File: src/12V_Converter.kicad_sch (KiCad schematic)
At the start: 37 parts, among them M4 CSD19534Q5A, M5 NVMFS6H836NLT1G, U2 LM5190RGYR (20V-50V)

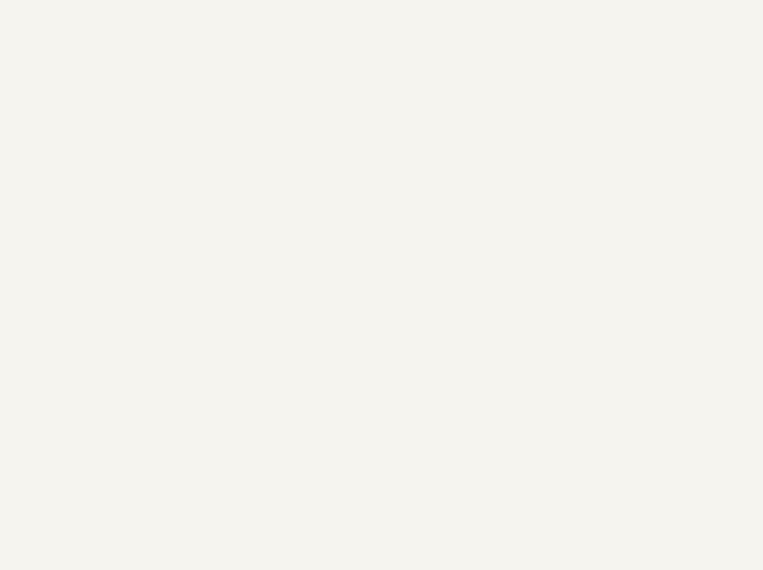
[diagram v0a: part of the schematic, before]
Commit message: Testing once again
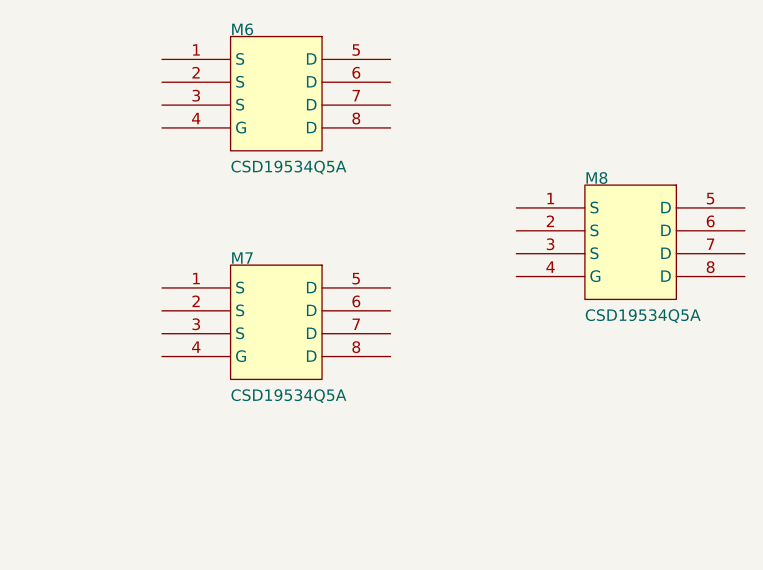
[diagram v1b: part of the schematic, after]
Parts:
- added M6, M7, M8: CSD19534Q5A, powerDristributionBoard-import-fps:DQJ8, symbol Schlib1:CSD19534Q5A

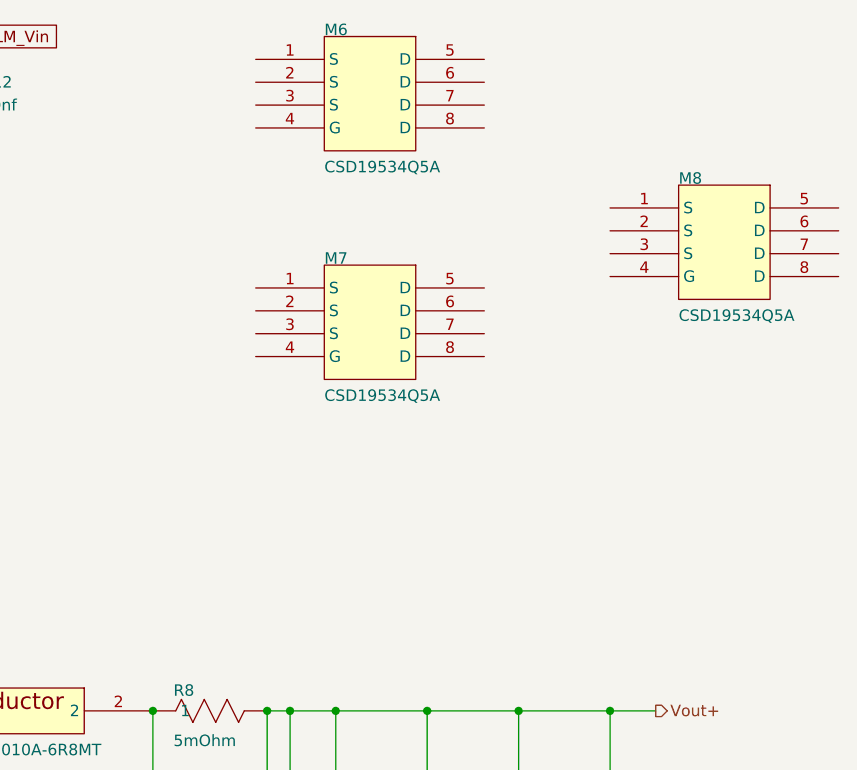
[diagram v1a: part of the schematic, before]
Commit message: Restored powerDistribution PCB files to commit 2fb1c3a
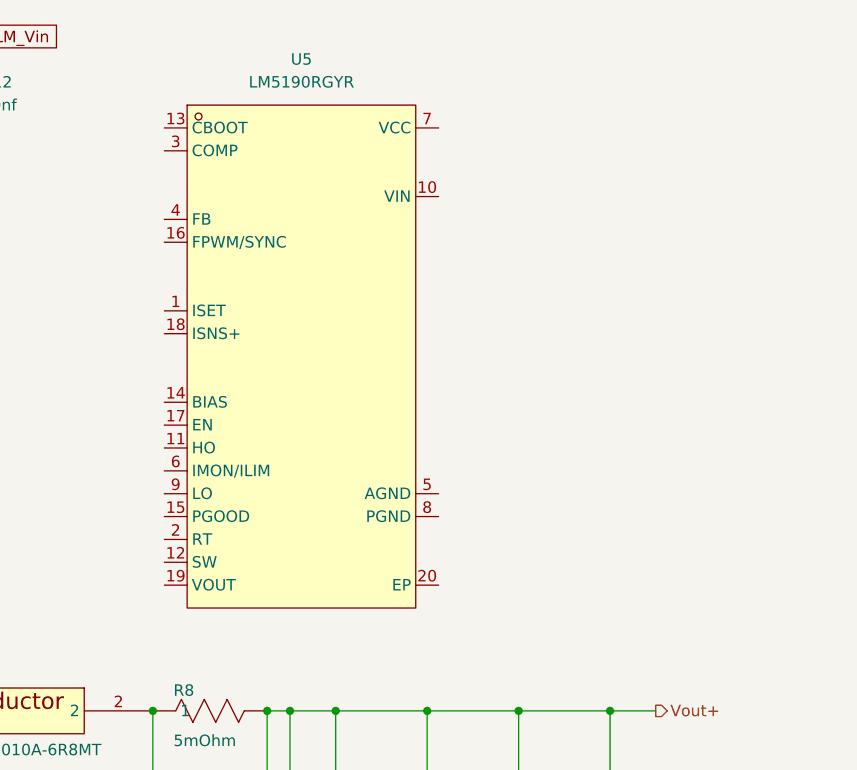
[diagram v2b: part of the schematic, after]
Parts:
- removed M6, M7, M8: CSD19534Q5A, powerDristributionBoard-import-fps:DQJ8, symbol Schlib1:CSD19534Q5A
- added U5: LM5190RGYR, EasyEDA:QFN-19_L4.5-W3.5-P0.50-BL-EP_TI_RGY, symbol EasyEDA:LM5190RGYR

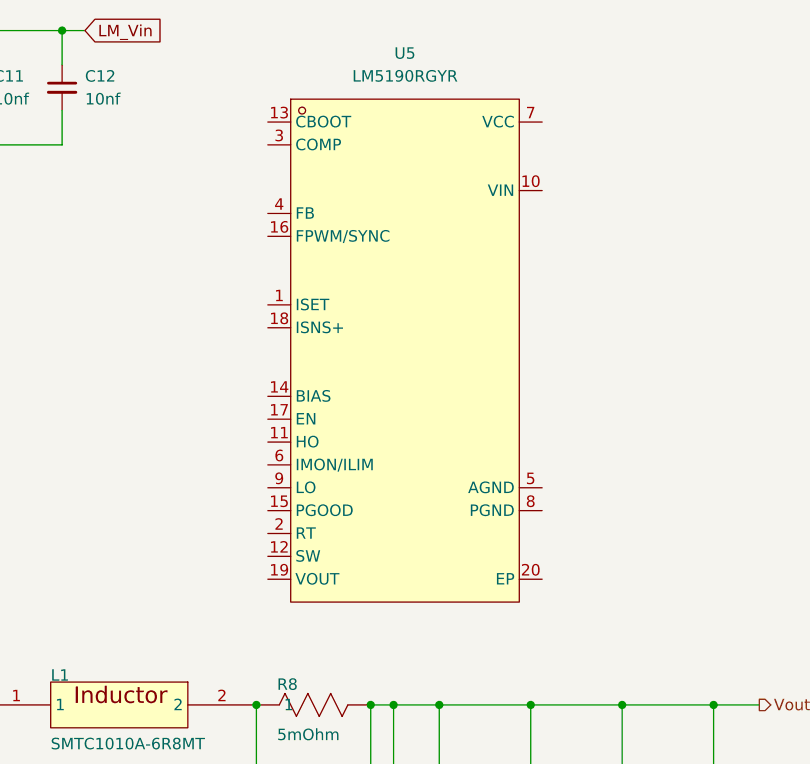
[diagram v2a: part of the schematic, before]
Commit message: Testing to merge again
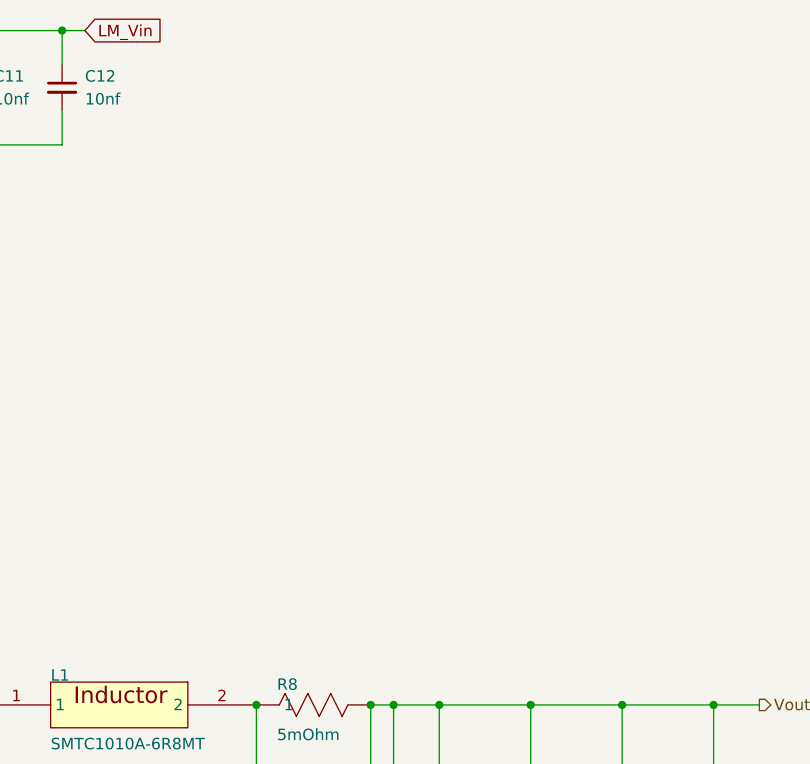
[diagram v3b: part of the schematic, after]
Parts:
- removed U5: LM5190RGYR, EasyEDA:QFN-19_L4.5-W3.5-P0.50-BL-EP_TI_RGY, symbol EasyEDA:LM5190RGYR
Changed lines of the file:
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@@
-	)
-	(symbol
-		(lib_id "EasyEDA:LM5190RGYR")
-		(at 222.25 57.15 0)
-		(unit 1)
-		(body_style 1)
-		(exclude_from_sim no)
-		(in_bom yes)
-		(on_board yes)
-		(in_pos_files yes)
-		(dnp no)
-		(fields_autoplaced yes)
-		(property "Reference" "U5"
-			(at 222.25 24.13 0)
-			(show_name no)
-			(do_not_autoplace no)
-			(effects
-				(font
-					(size 1.27 1.27)
-				)
-			)
-		)
-		(property "Value" "LM5190RGYR"
-			(at 222.25 26.67 0)
-			(show_name no)
-			(do_not_autoplace no)
-			(effects
-				(font
-					(size 1.27 1.27)
-				)
-			)
-		)
-		(property "Footprint" "EasyEDA:QFN-19_L4.5-W3.5-P0.50-BL-EP_TI_RGY"
-			(at 222.25 90.17 0)
-			(hide yes)
-			(show_name no)
-			(do_not_autoplace no)
-			(effects
-				(font
-					(size 1.27 1.27)
-				)
-			)
-		)
-		(property "Datasheet" "https://www.lcsc.com/datasheet/C43351172.pdf"
-			(at 222.25 92.71 0)
-			(hide yes)
-			(show_name no)
-			(do_not_autoplace no)
-			(effects
-				(font
-					(size 1.27 1.27)
-				)
-			)
-		)
-		(property "Description" ""
-			(at 222.25 57.15 0)
-			(hide yes)
-			(show_name no)
-			(do_not_autoplace no)
-			(effects
-				(font
-					(size 1.27 1.27)
-				)
-			)
-		)
-		(property "Manufacturer" "TI(德州仪器)"
-			(at 222.25 95.25 0)
-			(hide yes)
-			(show_name no)
-			(do_not_autoplace no)
-			(effects
-				(font
-					(size 1.27 1.27)
-				)
-			)
-		)
-		(property "MPN" "LM5190RGYR"
-			(at 222.25 97.79 0)
-			(hide yes)
-			(show_name no)
-			(do_not_autoplace no)
-			(effects
-				(font
-					(size 1.27 1.27)
-				)
-			)
-		)
-		(property "LCSC Part" "C43351172"
-			(at 222.25 100.33 0)
-			(hide yes)
-			(show_name no)
-			(do_not_autoplace no)
-			(effects
-				(font
-					(size 1.27 1.27)
-				)
-			)
-		)
-		(pin "8"
-		)
-		(pin "10"
-		)
-		(pin "2"
-		)
-		(pin "9"
-		)
-		(pin "4"
-		)
-		(pin "6"
-		)
-		(pin "7"
-		)
-		(pin "5"
-		)
-		(pin "11"
-		)
-		(pin "12"
-		)
-		(pin "13"
-		)
-		(pin "14"
-		)
-		(pin "15"
-		)
-		(pin "16"
-		)
-		(pin "17"
-		)
-		(pin "18"
-		)
-		(pin "19"
-		)
-		(pin "20"
-		)
-		(pin "1"
-		)
-		(pin "3"
-		)
-		(instances
-			(project "powerDristributionBoard"
-				(path "/501e9f3f-9bfa-47dd-b56d-5fd6974f0d03/8cad4ca2-ba0b-4eb3-ba1b-4233b97b1d3e"
-					(reference "U5")
-					(unit 1)
-				)
-			)
-		)
 	)
 	(symbol
